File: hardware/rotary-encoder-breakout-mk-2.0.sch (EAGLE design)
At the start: 7 parts, among them U1 ROTARY_ENCODER_SWITCH, U2 Tiny85

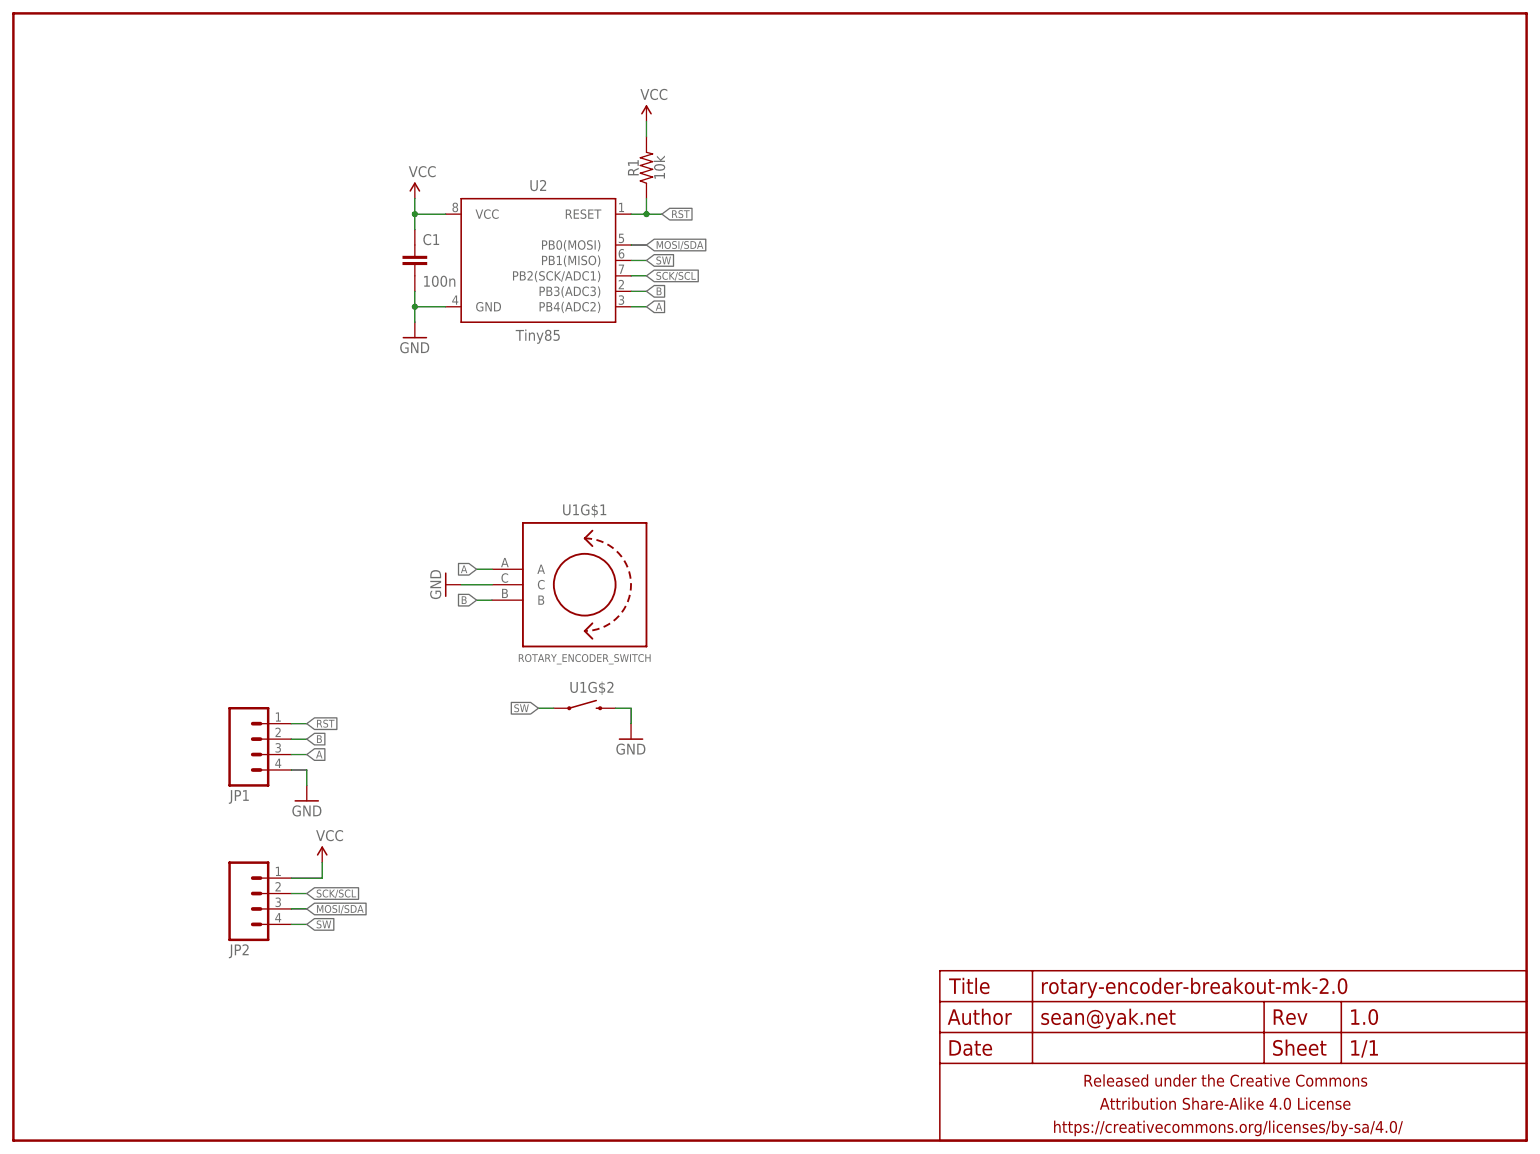
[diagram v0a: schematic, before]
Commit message: have some boards, dawg
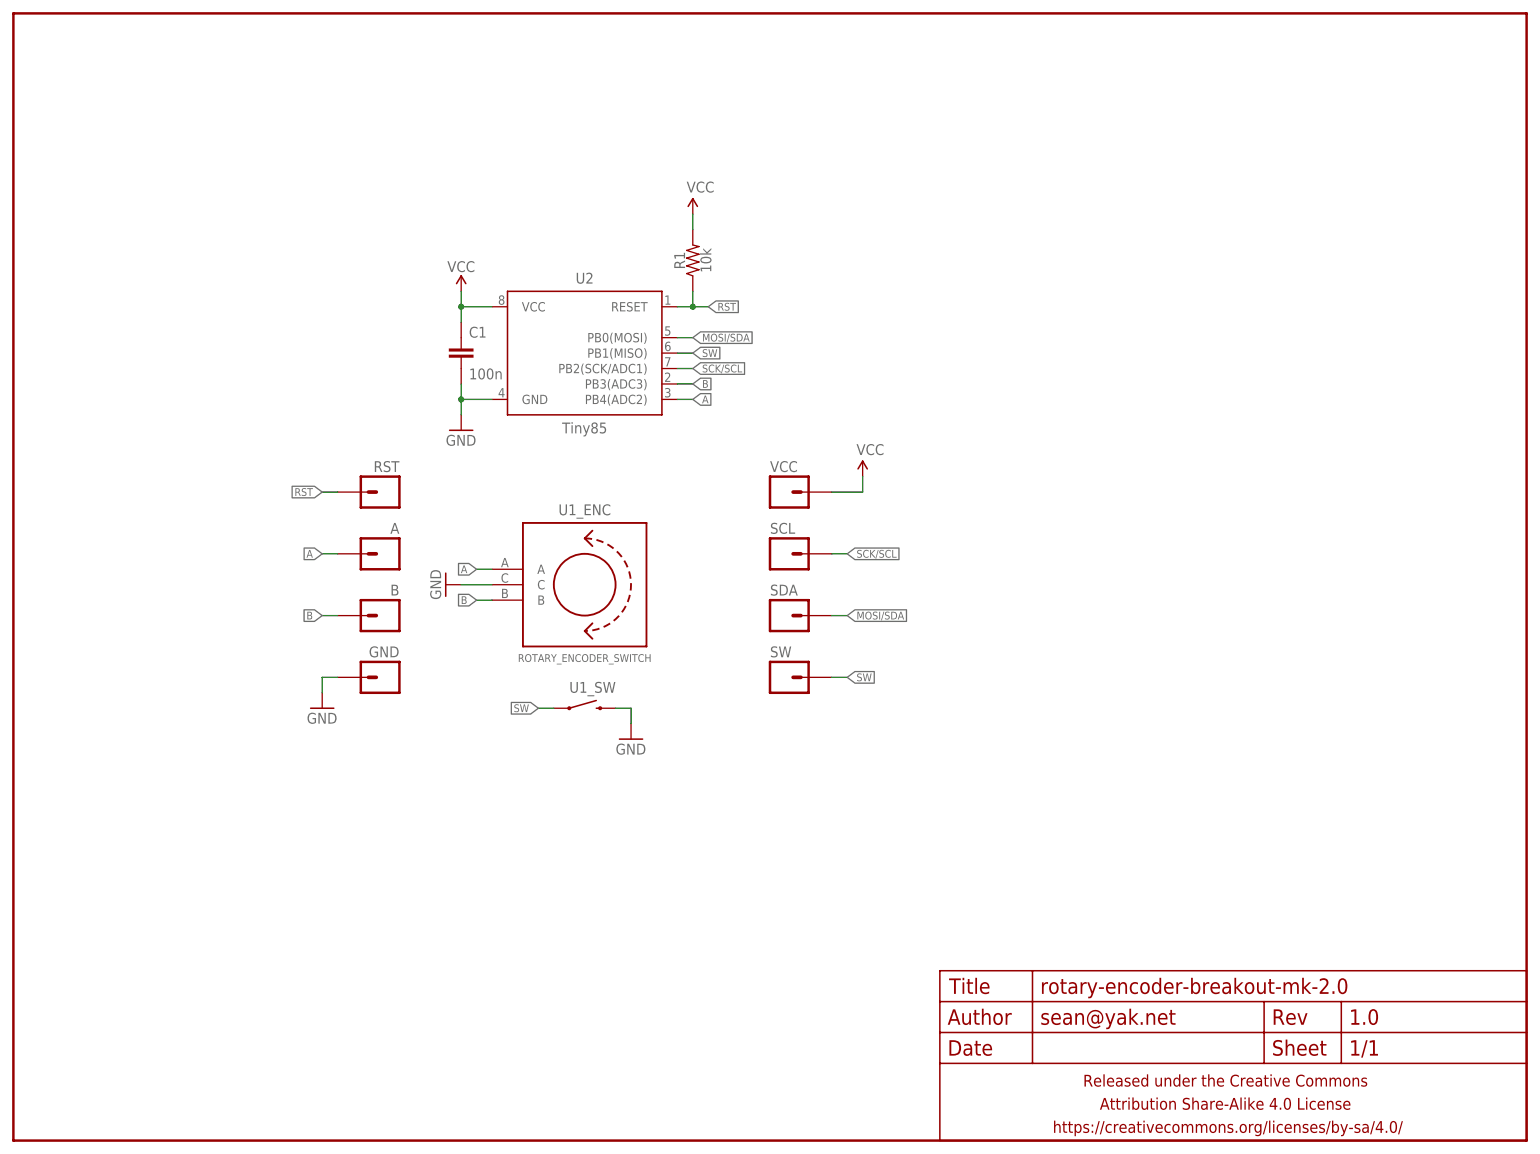
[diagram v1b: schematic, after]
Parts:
- removed JP1, JP2: M04PTH, A_butts:M04PTH
- removed U1: ROTARY_ENCODER_SWITCH, A_butts:ROTARY_ENCODER_SWITCH
- added A, B, GND, RST, SCL, SDA, SW, VCC: M01PTH-1MM, a_parts:M01PTH-1MM
- added U1_: ROTARY_ENCODER_SWITCH, a_parts:ROTARY_ENCODER_SWITCH
- C1: device A_butts:CAPACITOR-CERAMICC0805 -> a_parts:CAPACITOR-CERAMICC0603-TIGHTER
- R1: device A_butts:RESISTORR0805 -> a_parts:RESISTORR0603-TIGHTER
- U2: device A_butts:ATTINY45TINY85-20-SOICW -> a_parts:ATTINY45TINY85-20-SOICW
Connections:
- net A: now also A.1, U1_ENC.A; no longer JP1.3, U1G$1.A
- net B: now also B.1, U1_ENC.B; no longer JP1.2, U1G$1.B
- net GND: now also GND.1, U1_ENC.C, U1_SW.2; no longer JP1.4, U1G$1.C, U1G$2.2
- net MOSI/SDA: now also SDA.1; no longer JP2.3
- net RST: now also RST.1; no longer JP1.1
- net SCK/SCL: now also SCL.1; no longer JP2.2
- net SW: now also SW.1, U1_SW.1; no longer JP2.4, U1G$2.1
- net VCC: now also VCC.1; no longer JP2.1
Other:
- moved on the sheet: C1, R1, U2
